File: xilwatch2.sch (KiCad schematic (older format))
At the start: 1 part

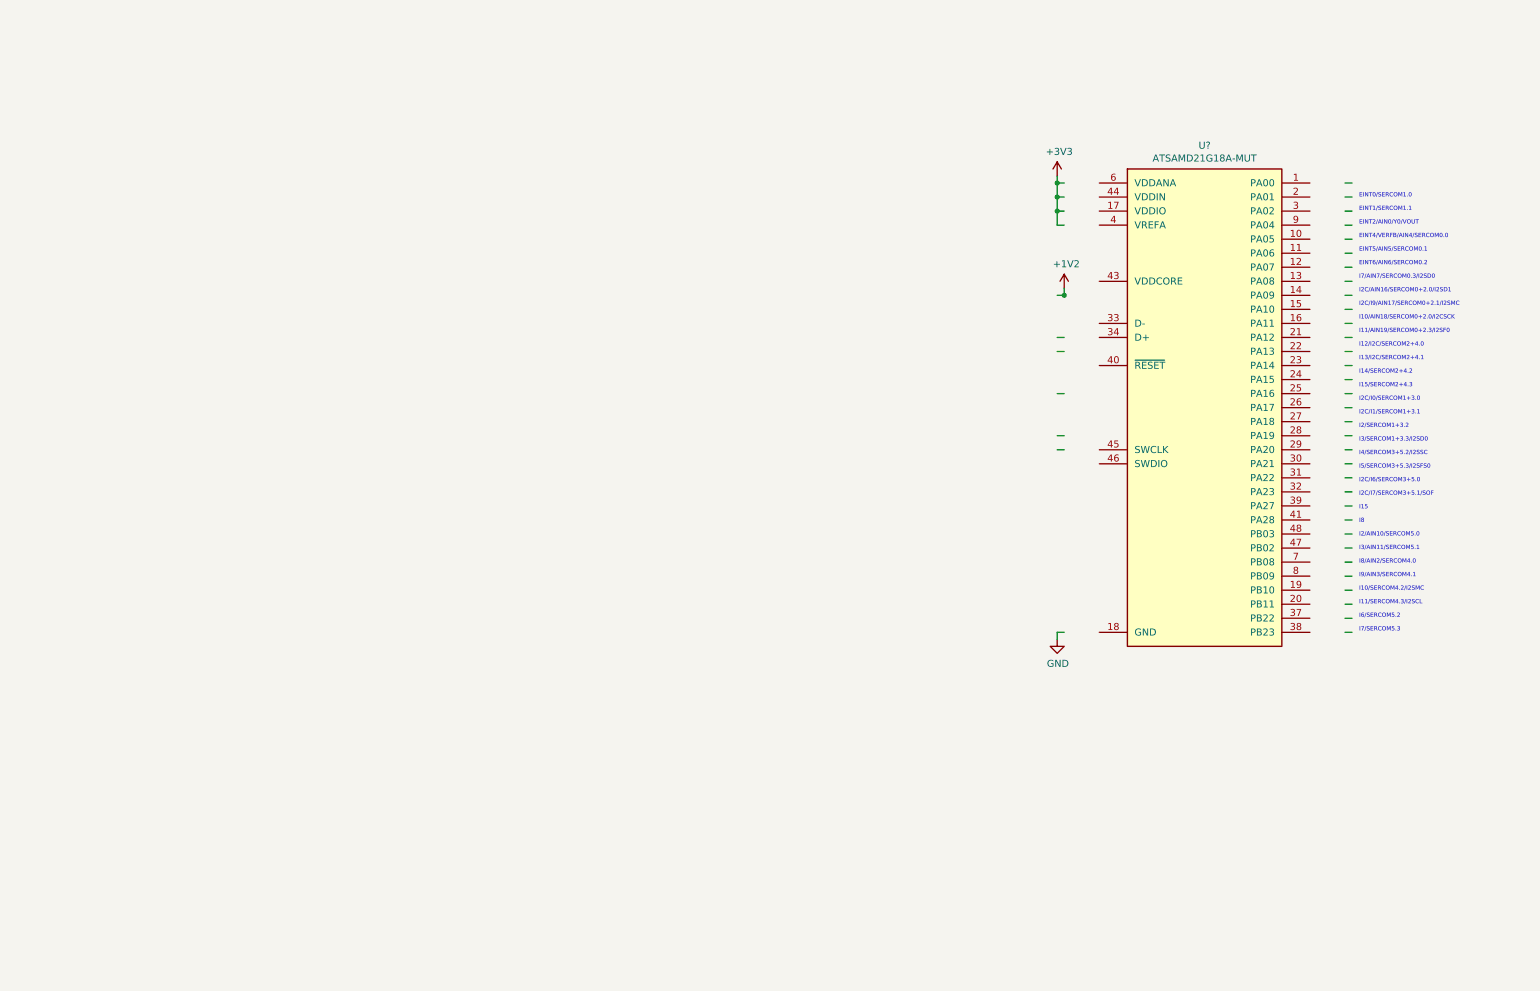
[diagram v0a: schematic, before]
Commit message: More work, mostly copied from rev1
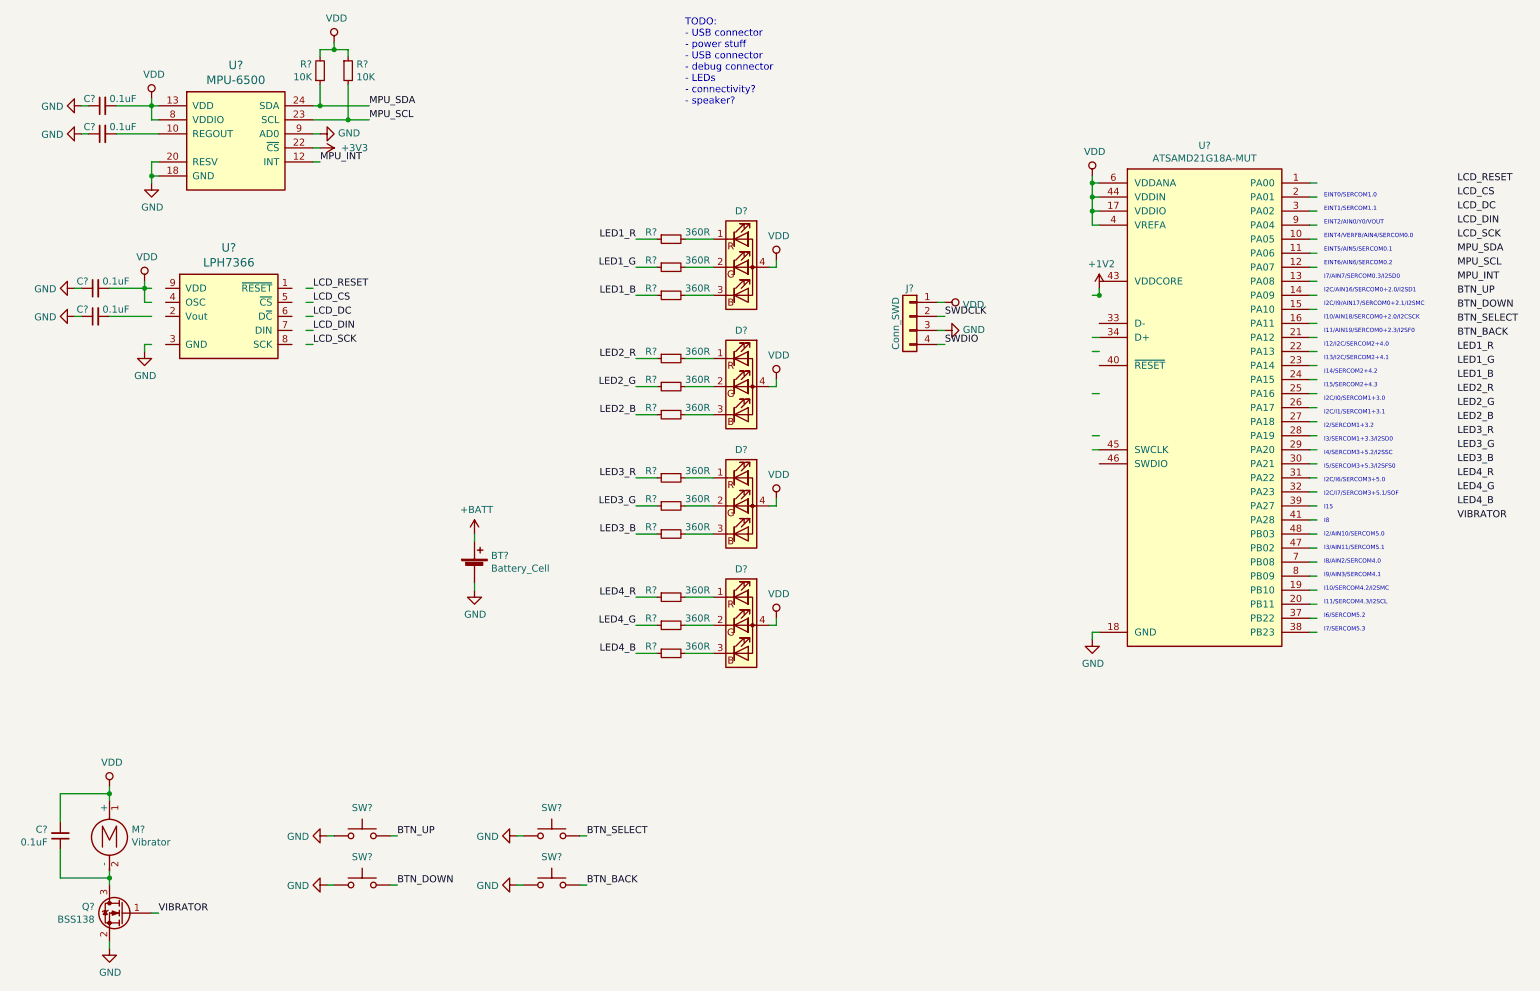
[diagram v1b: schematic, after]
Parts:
- added BT?: Battery_Cell, symbol Device:Battery_Cell
- added C? (x5): 0.1uF, symbol Device:C_Small
- added D?: LED_TopLeft, symbol Device_Extra:LED_RGBA
- added D?: LED_TopRight, symbol Device_Extra:LED_RGBA
- added D?: LED_BottomLeft, symbol Device_Extra:LED_RGBA
- added D?: LED_BottomRight, symbol Device_Extra:LED_RGBA
- added J?: Conn_SWD, symbol Connector_Generic:Conn_01x04
- added M?: Vibrator, symbol Motor:Motor_DC
- added Q?: BSS138, Package_TO_SOT_SMD:SOT-23, symbol Transistor_FET:BSS138
- added R? (x2): 10K, symbol Device:R_Small
- added R? (x12): 360R, symbol Device:R_Small
- added SW?: Btn_Up, symbol Switch:SW_Push
- added SW?: Btn_Select, symbol Switch:SW_Push
- added SW?: Btn_Down, symbol Switch:SW_Push
- added SW?: Btn_Back, symbol Switch:SW_Push
- added U?: MPU-6500, symbol Sensor_Motion_Extra:MPU-6500
- added U?: LPH7366, symbol Display_Graphic_Extra:LPH7366
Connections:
- net labels added: +BATT, BTN_BACK, BTN_DOWN, BTN_SELECT, BTN_UP, LCD_CS, LCD_DC, LCD_DIN, LCD_RESET, LCD_SCK, LED1_B, LED1_G, LED1_R, LED2_B, LED2_G, LED2_R, LED3_B, LED3_G, LED3_R, LED4_B, LED4_G, LED4_R, MPU_INT, MPU_SCL, MPU_SDA, SWDCLK, SWDIO, VDD, VIBRATOR
- wire segments 50 -> 147
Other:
- note added: "TODO:\n- USB connector\n- power stuff\n- USB connector\n- debug connector\n- LEDs\n- connectivity?\n- speaker?"
